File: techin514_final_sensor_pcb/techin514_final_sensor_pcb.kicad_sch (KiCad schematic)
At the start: 14 parts, among them J1 SW1, J2 J_BAT, J4 J_LDO, J5 J_MOTOR, J6 J_IMU, J7 J_PWR, U3 ULN2003

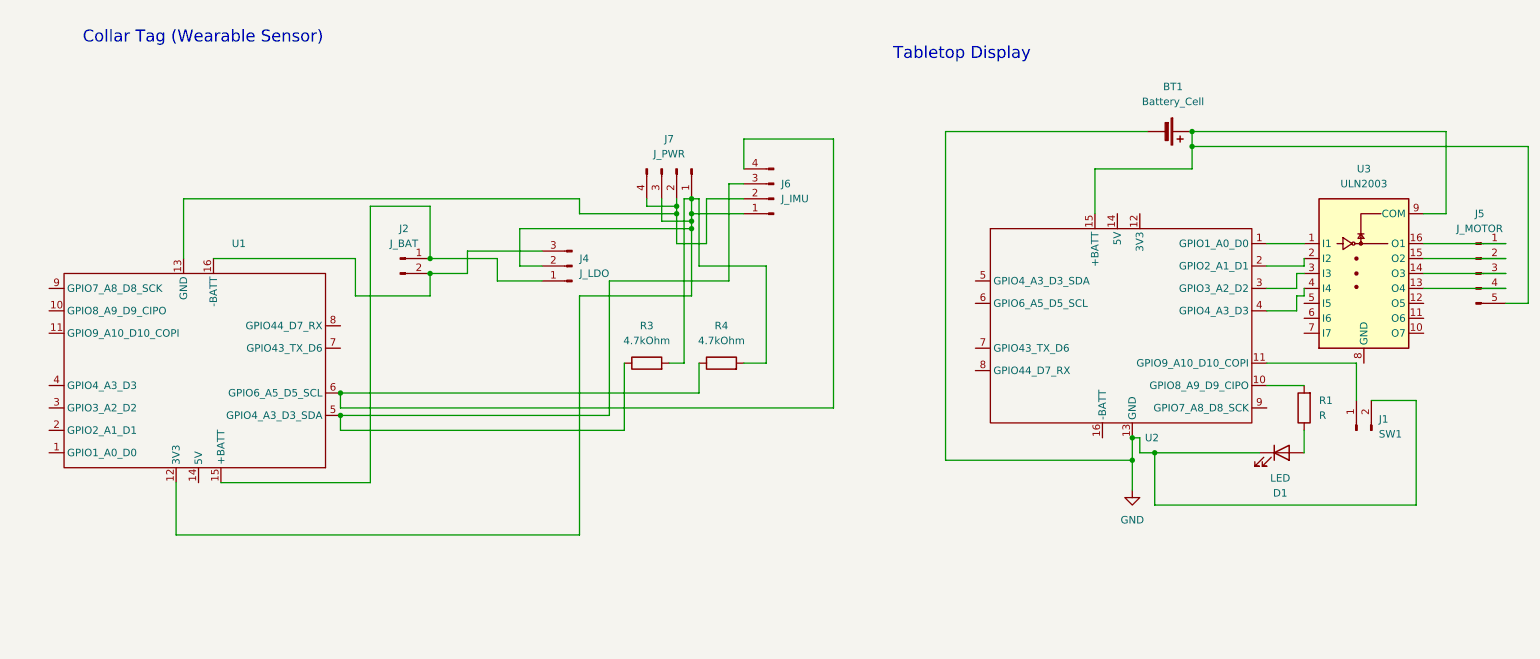
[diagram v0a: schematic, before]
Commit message: update code
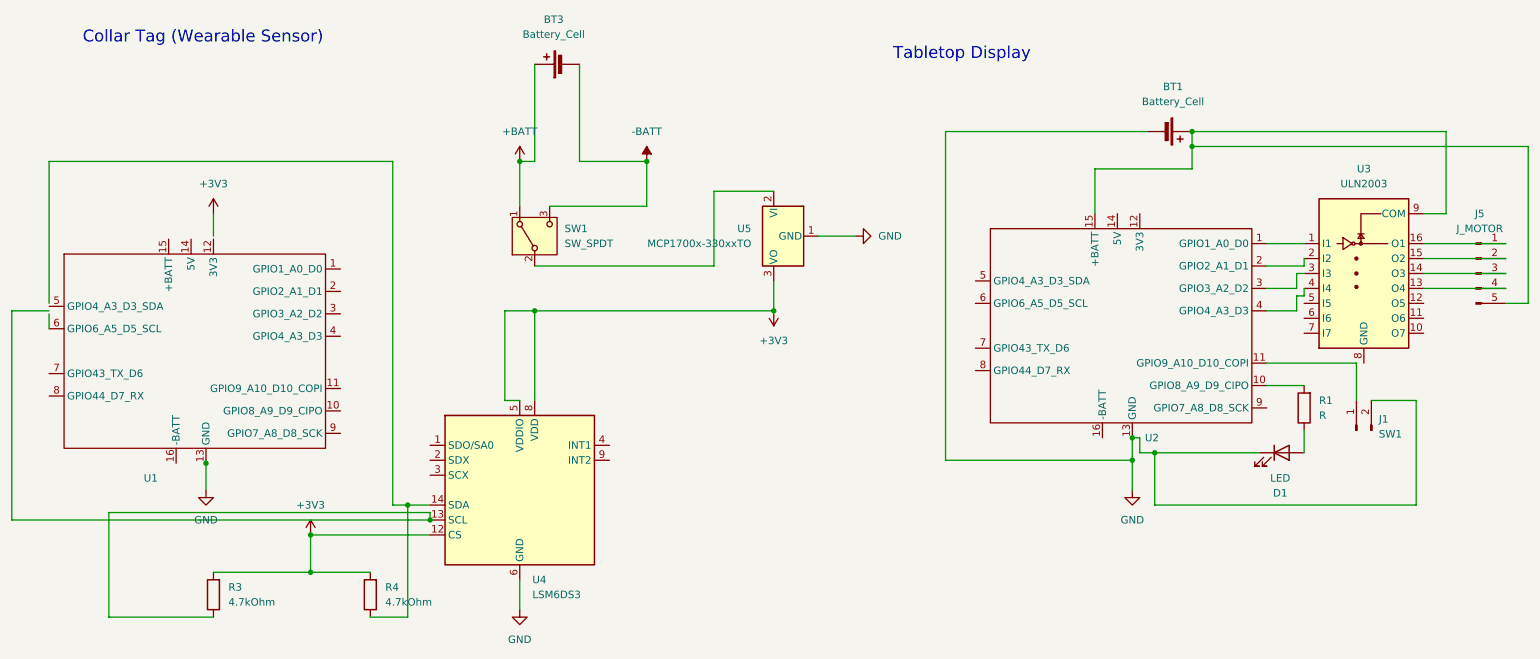
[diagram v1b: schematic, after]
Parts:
- removed J2: J_BAT, Connector_PinHeader_2.54mm:PinHeader_1x02_P2.54mm_Vertical, symbol Connector:Conn_01x02_Pin
- removed J4: J_LDO, Connector_PinHeader_2.54mm:PinHeader_1x02_P2.54mm_Vertical, symbol Connector:Conn_01x03_Pin
- removed J6: J_IMU, Connector_PinHeader_2.54mm:PinHeader_1x04_P2.54mm_Vertical, symbol Connector:Conn_01x04_Pin
- removed J7: J_PWR, Connector_PinHeader_2.54mm:PinHeader_1x02_P2.54mm_Vertical, symbol Connector:Conn_01x04_Pin
- added BT3: Battery_Cell, symbol Device:Battery_Cell
- added SW1: SW_SPDT, Connector_PinHeader_2.54mm:PinHeader_1x03_P2.54mm_Vertical, symbol Switch:SW_SPDT
- added U4: LSM6DS3, Connector_PinHeader_2.54mm:PinHeader_1x05_P2.54mm_Vertical, symbol Sensor_Motion:LSM6DS3
- added U5: MCP1700x-330xxTO, Connector_PinHeader_2.54mm:PinHeader_1x03_P2.54mm_Vertical, symbol Regulator_Linear:MCP1700x-330xxTO
- J1: footprint Connector_PinHeader_2.54mm:PinHeader_1x02_P2.54mm_Vertical -> Button_Switch_THT:SW_Slide-03_Wuerth-WS-SLTV_10x2.5x6.4_P2.54mm
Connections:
- net GND: now also U1.13 (GND), U4.6 (GND), U4.7 (GND), U5.1 (GND)
- net +3V3: now reaches R3.2, R4.2
- net +3V3: now also U4.12 (CS), U4.5 (VDDIO), U4.8 (VDD), U5.3 (VO); no longer U1.12 (3V3)
- net at R3.1: now also U4.13 (SCL); no longer U1.5 (GPIO4_A3_D3_SDA)
- net at R4.1: now also U4.14 (SDA); no longer U1.6 (GPIO6_A5_D5_SCL)
- new net: SW1.2 (B), U5.2 (VI)
- new net +BATT: BT3.1 (+), SW1.1 (A)
- new net -BATT: BT3.2 (-), SW1.3 (C)
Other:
- moved on the sheet: R3, R4, U1
